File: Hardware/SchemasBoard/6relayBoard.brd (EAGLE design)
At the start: 53.1 x 41.8 mm, 47 parts, among them IC1 LNK304, IC3 MC33269ST-3.3T3, K1 FRS1B, K2 FRS1B, K3 FRS1B, K4 FRS1B, K5 FRS1B, K6 FRS1B, T1 BC846, T2 BC846, T3 BC846, T4 BC846, T5 BC846, T6 BC846

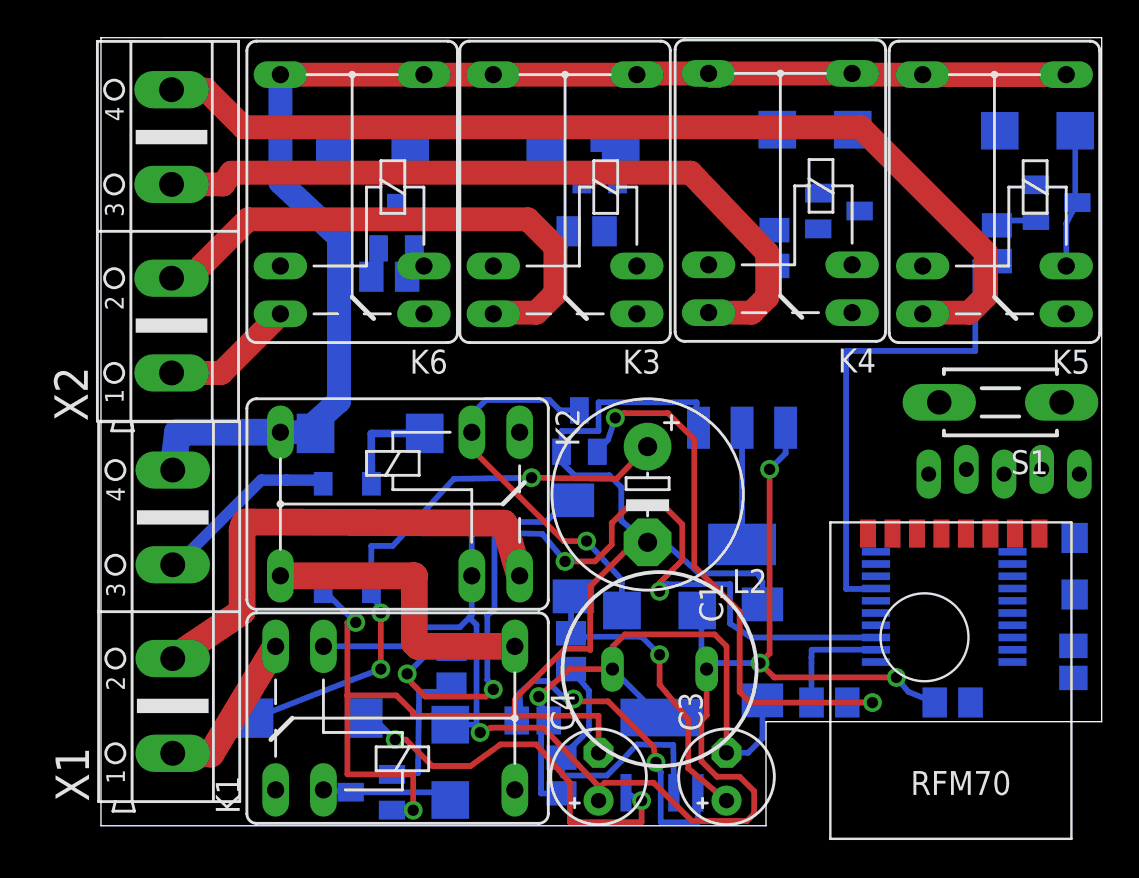
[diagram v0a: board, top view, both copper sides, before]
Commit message: aaa
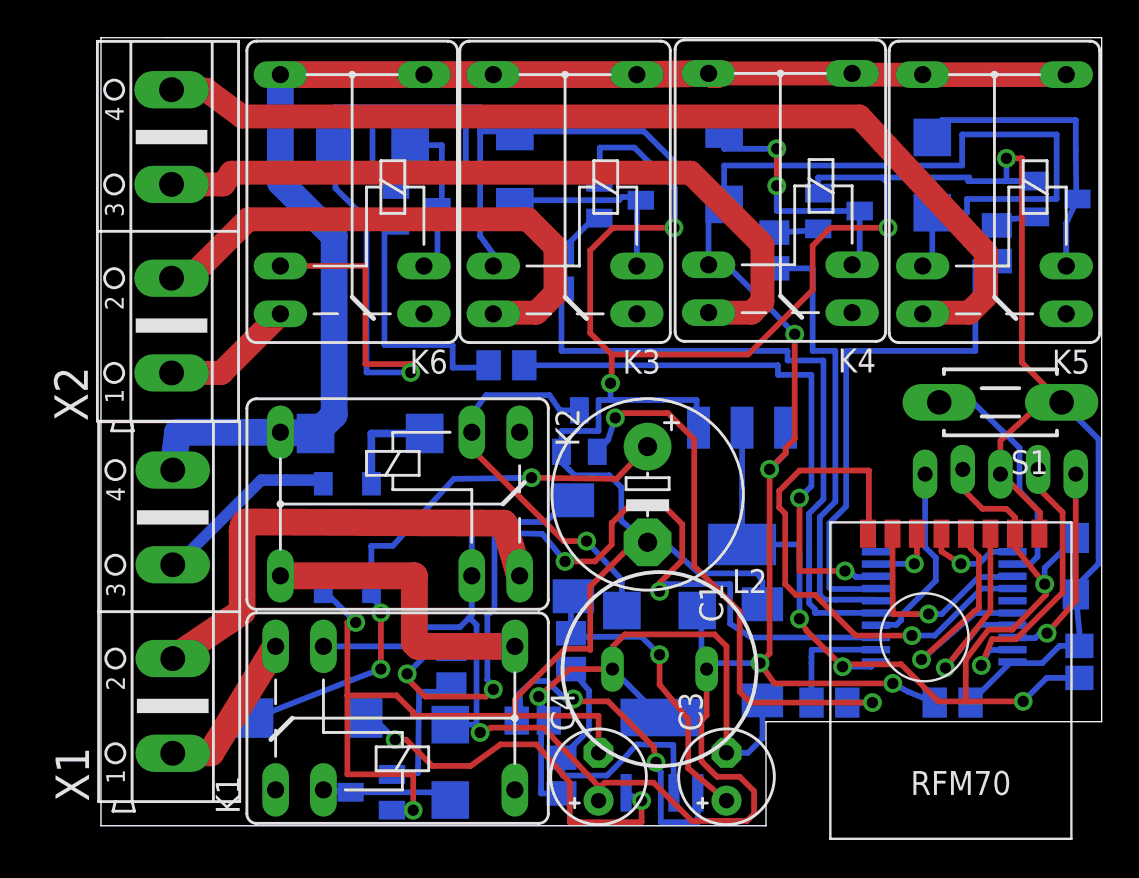
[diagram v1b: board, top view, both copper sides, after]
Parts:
- moved R11 7.80 mm to (20.4, 24.4)
- moved D5 6.06 mm to (43.0, 34.5), turned to 90 degrees
- moved D6 5.21 mm to (31.9, 35.0), turned to 90 degrees
- moved D7 3.70 mm to (20.8, 34.9), turned to 270 degrees
- moved R10 2.55 mm to (23.2, 29.5), turned to 90 degrees
- moved T5 2.41 mm to (26.4, 33.2), turned to 90 degrees
- moved T6 1.53 mm to (15.6, 32.8), turned to 90 degrees
- moved C5 0.32 mm to (50.8, 8.70)
- moved T3 0.19 mm to (49.6, 33.3)
- moved U$3 0.19 mm to (46.6, 18.7)
- moved R9 0.13 mm to (34.6, 30.5)
- moved C6 0.06 mm to (50.6, 13.8)
- turned D8 to 180 degrees
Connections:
- net N$27: now also K3.1
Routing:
- net GND: track 74.0 -> 199.4 mm, vias 2 -> 6
- net N$27: track 85.2 -> 198.8 mm, vias 4 -> 6
- net N$17: track 6.20 -> 52.8 mm, vias 0 -> 4
- net N$45: track 0.00 -> 34.9 mm
- net N$29: track 0.00 -> 30.7 mm, vias 0 -> 2
- net N$21: track 0.00 -> 27.9 mm, vias 0 -> 1
- net N$46: track 0.00 -> 24.1 mm
- net N$18: track 0.00 -> 15.4 mm, vias 0 -> 1
- net N$31: track 0.00 -> 14.8 mm, vias 0 -> 2
- net N$20: track 0.00 -> 14.6 mm, vias 0 -> 1
- net N$44: track 0.00 -> 13.8 mm
- net N$5: track 0.00 -> 12.9 mm
- net N$16: track 0.00 -> 12.7 mm, vias 0 -> 1
- net N$12: track 0.00 -> 11.5 mm, vias 0 -> 1
- net N$19: track 0.00 -> 11.0 mm, vias 0 -> 1
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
